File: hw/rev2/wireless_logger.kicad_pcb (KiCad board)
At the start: 4 copper layers, 98 parts, among them J1 FCI 10118194, J3 SSD1306_SER, J4 SWD_10PIN, Q1 2N7002P, Q2 2N7002P, U1 MT29FXX01A, U10 CC2541, U11 STM32F40X_BGA176, U2 MAG3110, U3 MMA8452Q, U4 LPS331AP, U5 L3GD20, U6 MCP111T-315, U7 BQ24095, U8 TPS62698, U9 CC1101, X1 FA-128 26.0000MF10Z-W3, X2 9HT10-32.768KBZF-T, X3 FA-128 32.0000MF20X-K3, X4 XRCGB25M000F0L00R0, X5 9HT10-32.768KBZF-T

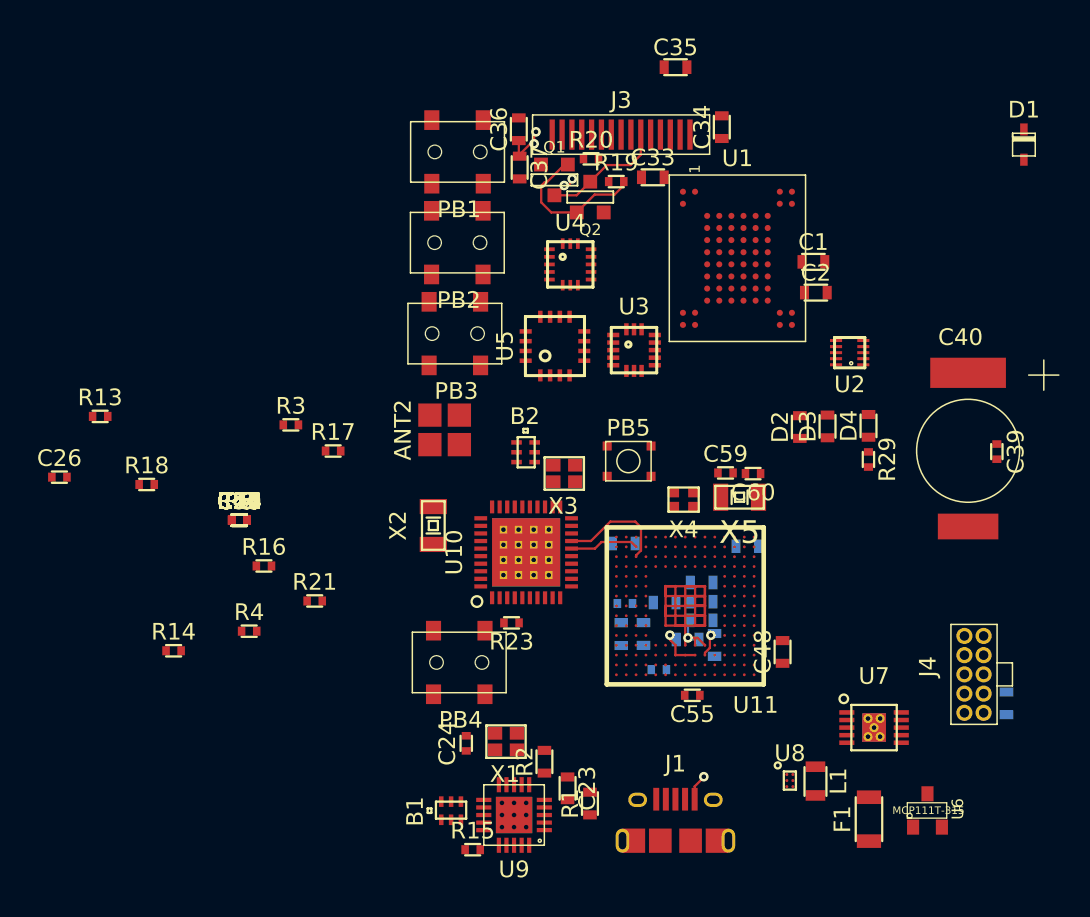
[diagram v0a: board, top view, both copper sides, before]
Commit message: Uhhhh, secondary interconnect assignment and a LOT of routing
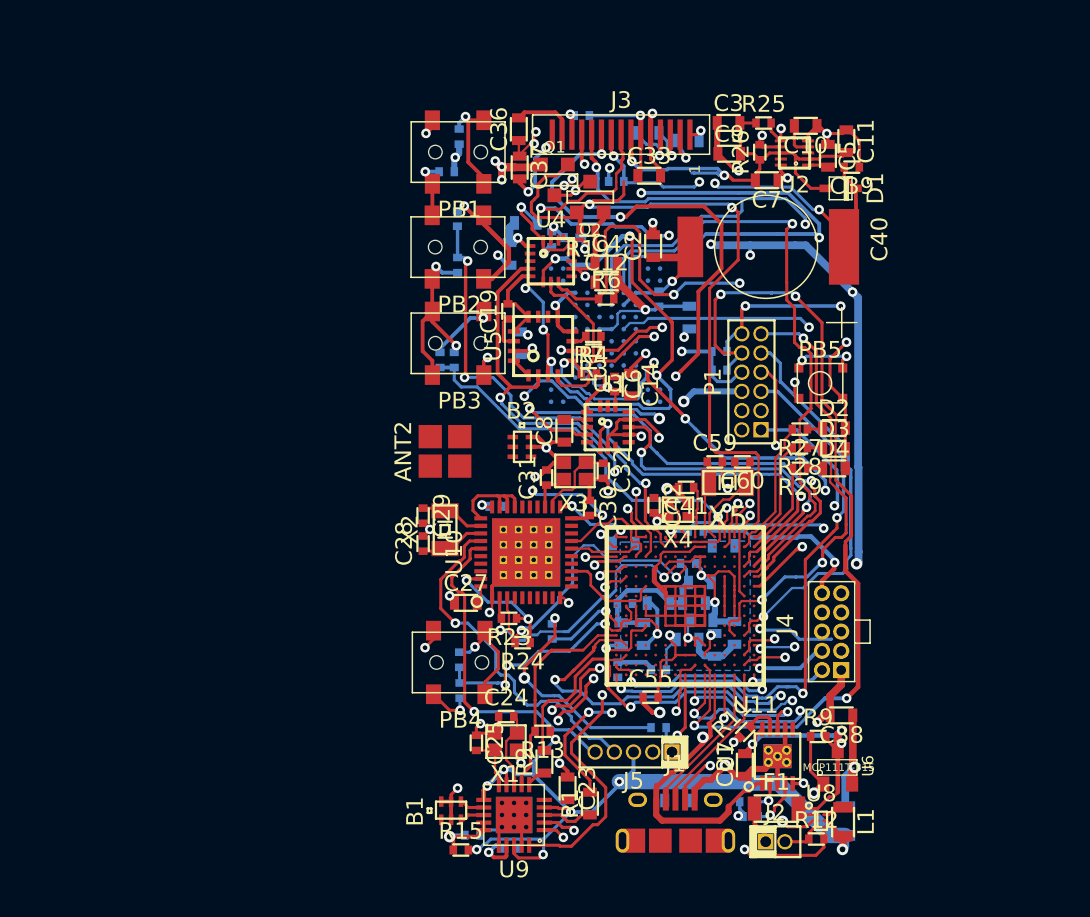
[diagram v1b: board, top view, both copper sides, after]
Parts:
- added C10: 100n, SMD0603, F.Cu at (195.9, 111.4)
- added C11: 100n, SMD0603, F.Cu at (198.6, 112.4)
- added C12: 100n, SMD0603, F.Cu at (182.8, 121.7)
- added C13: 10n, SMD0402, B.Cu at (179.1, 118.9)
- added C14: 2.2u, SMD0603, F.Cu at (184.4, 128.5)
- added C15: 100n, SMD0603, B.Cu at (177.0, 125.7)
- added C16: 100p, SMD0402, B.Cu at (186.2, 122.8)
- added C17: 100n, SMD0603, B.Cu at (177.4, 117.8)
- added C18: 1u, SMD0603, B.Cu at (176.4, 119.8)
- added C19: 10n, SMD0402, F.Cu at (176.2, 123.6)
- added C20: 2.2u, SMD0603, B.Cu at (187.4, 155.9)
- added C21: 2.2u, SMD0603, F.Cu at (191.9, 153.6)
- added C22: 10u, SMD0805, B.Cu at (198.5, 157.3)
- added C27: 1u, SMD0603, F.Cu at (173.5, 142.9)
- added C28: 15p, SMD0402, F.Cu at (170.6, 139.0)
- added C29: 15p, SMD0402, F.Cu at (170.6, 137.1)
- added C3: 2.2u, SMD0603, F.Cu at (190.8, 111.2)
- added C30: 1n, SMD0402, F.Cu at (181.6, 136.6)
- added C31: 12p, SMD0402, F.Cu at (178.8, 134.6)
- added C32: 12p, SMD0402, F.Cu at (182.5, 134.1)
- added C4: 100n, SMD0603, F.Cu at (182.7, 120.5)
- added C5: 100n, SMD0603, F.Cu at (197.4, 113.3)
- added C6: 100p, SMD0402, F.Cu at (183.3, 128.4)
- added C61: 10n, SMD0402, B.Cu at (172.2, 114.4)
- added C62: 10n, SMD0402, B.Cu at (172.9, 120.6)
- added C63: 10n, SMD0402, B.Cu at (172.7, 126.8)
- added C64: 10n, SMD0402, B.Cu at (173.1, 148.7)
- added C7: 1u, SMD0603, F.Cu at (193.3, 115.0)
- added C8: 100n, SMD0603, F.Cu at (180.0, 131.5)
- added C9: 100n, SMD0603, F.Cu at (190.9, 113.2)
- added J2: CONN_2, HDR_2X1_50MIL, F.Cu at (193.9, 158.7)
- added J5: CONN_5, HDR_5X1_50MIL, F.Cu at (184.5, 152.7)
- added P1: CONN_6X2, HDR_6X2_50MIL, F.Cu at (192.3, 128.3)
- added R30: 470k, SMD0402, B.Cu at (173.0, 112.1)
- added R31: 470k, SMD0402, B.Cu at (172.9, 117.5)
- added R32: 470k, SMD0402, B.Cu at (171.8, 126.8)
- added R33: 470k, SMD0402, B.Cu at (173.0, 146.6)
- added R34: 10k, SMD0402, B.Cu at (190.2, 126.3)
- added R35: 10k, SMD0402, B.Cu at (190.2, 127.5)
- C1, C26, C34, C35, C48, C54, C58, R10, R14, R16, R17, R18, R20, R21, R22, R5, R8, U1: moved to B.Cu
- C38: moved to F.Cu
- moved R12 43.6 mm to (196.6, 158.5)
- moved R25 43.5 mm to (193.1, 111.2)
- moved R26 42.1 mm to (192.9, 113.1), turned to 90 degrees
- moved R9 40.8 mm to (196.7, 151.7)
- moved R10 39.0 mm to (192.3, 157.0)
- moved R8 38.4 mm to (192.1, 156.0)
- moved R27 37.5 mm to (195.5, 131.4), turned to 180 degrees
- moved R28 37.3 mm to (195.5, 132.6), turned to 180 degrees
- moved R21 36.6 mm to (181.1, 110.7), turned to 180 degrees
- moved R11 36.2 mm to (191.9, 151.4), turned to 45 degrees
- moved C26 36.1 mm to (173.9, 158.2), turned to 180 degrees
- moved R13 35.9 mm to (178.5, 151.4), turned to 180 degrees
- moved R22 30.2 mm to (188.7, 138.1)
- moved R4 29.9 mm to (181.9, 125.3), turned to 180 degrees
- moved C54 29.8 mm to (188.1, 140.3)
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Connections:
- net N-00000242 renamed /Bluetooth/BT_ANT_DN
- net N-00000243 renamed /Bluetooth/BT_ANT_DP
- net N-00000244 renamed /Bluetooth/BT_ANT_SE
- C1 pad 2: VDD -> V3
- C2 pad 2: VDD -> V3
- C38 pad 2: N-0000078 -> V3
- C45 pad 2: VDD -> V3
- C46 pad 2: VDD -> V3
- C47 pad 2: VDD -> V3
- C48 pad 2: VDD -> V3
- C49 pad 2: VDD -> V3
- C50 pad 2: VDD -> V3
- C51 pad 2: VDD -> V3
- C52 pad 2: VDD -> V3
- C53 pad 2: VDD -> V3
- C54 pad 2: VDD -> V3
- C55 pad 2: VDD -> V3
- C56 pad 2: VDD -> V3
- C57 pad 2: VDD -> V3
- C58 pad 2: VDD -> V3
- D1 pad 1: VDD -> V3
- J3 pad 10: (no net) -> /STM32F4/OLED_nD/C
- J3 pad 7: VDD -> V3
- J3 pad 8: (no net) -> /STM32F4/OLED_nCS
- J4 pad 1: N-0000078 -> V3
- PB1 pad 1: /STM32F4/EXTI5 -> N-0000047
- PB2 pad 1: /STM32F4/EXTI6 -> N-0000046
- PB3 pad 1: /STM32F4/EXTI7 -> N-0000045
- PB4 pad 1: /STM32F4/EXTI8 -> N-0000044
- R13 pad 1: VDD -> V3
- R15 pad 2: VDD -> V3
- R16 pad 1: /STM32F4/BT_NRESET -> /Bluetooth/RF_RESET_N_LOCAL
- R17 pad 1: /STM32F4/BT_NRESET -> /Bluetooth/RF_RESET_N_LOCAL
- R20 pad 1: GND -> /OLED/OLED_GND
- R23 pad 1: VDD -> V3
- R24 pad 1: VDD -> V3
- R25 pad 1: VDD -> V3
- R26 pad 1: VDD -> V3
- R27 pad 2: (no net) -> /STM32F4/LED1
- R28 pad 2: (no net) -> /STM32F4/LED2
- R29 pad 2: (no net) -> /STM32F4/LED3
- R5 pad 1: VDD -> V3
- R6 pad 2: VDD -> V3
- R7 pad 2: VDD -> V3
- U1 pad D3: VDD -> V3
- U1 pad G5: VDD -> V3
- U1 pad G6: VDD -> V3
- U1 pad J8: VDD -> V3
- U1 pad K7: (no net) -> /STM32F4/FLASH_nCS
- U10 pad 10: VDD -> V3
- U10 pad 13: (no net) -> /STM32F4/EXTI2
- U10 pad 20: /STM32F4/BT_NRESET -> /Bluetooth/RF_RESET_N_LOCAL
- U10 pad 21: VDD -> V3
- U10 pad 24: VDD -> V3
- U10 pad 27: VDD -> V3
- U10 pad 28: VDD -> V3
- U10 pad 29: VDD -> V3
- U10 pad 31: VDD -> V3
- U10 pad 39: VDD -> V3
- U10 pad GND: (no net) -> GND
- U11 pad A1: (no net) -> /STM32F4/LED2
- U11 pad A2: (no net) -> /STM32F4/LED3
- U11 pad A4: (no net) -> /Sensors/ACC_INT1
- U11 pad A6: (no net) -> /STM32F4/GYRO_nCS
- U11 pad B1: (no net) -> /OLED/EN
- U11 pad B11: (no net) -> /STM32F4/UART2_RX
- U11 pad B2: (no net) -> /STM32F4/LED1
- U11 pad B5: (no net) -> /STM32F4/FLASH_nCS
- U11 pad B7: (no net) -> /Sensors/PRS_SPI_nCS
- U11 pad C11: (no net) -> /STM32F4/UART2_TX
- U11 pad C5: VDD -> V3
- U11 pad C6: VDD -> V3
- U11 pad C7: VDD -> V3
- U11 pad C8: VDD -> V3
- U11 pad C9: VDD -> V3
- U11 pad D1: (no net) -> /STM32F4/OLED_nCS
- U11 pad D2: (no net) -> /STM32F4/OLED_nRES
- U11 pad F14: (no net) -> /STM32F4/I2C3_SDA
- U11 pad F15: (no net) -> /STM32F4/I2C3_SCL
- U11 pad F3: VDD -> V3
- U11 pad G13: VDD -> V3
- U11 pad G14: (no net) -> /STM32F4/REG_nUSB_CONN
- U11 pad G15: (no net) -> /STM32F4/REG_nCHG
- U11 pad G3: VDD -> V3
- U11 pad H13: VDD -> V3
- U11 pad H15: (no net) -> /Power/MODE
- U11 pad J12: VDD -> V3
- U11 pad J13: VDD -> V3
- U11 pad K1: (no net) -> /STM32F4/EXTI7
- U11 pad K4: VDD -> V3
- U11 pad M3: (no net) -> /STM32F4/EXTI1
- U11 pad M6: (no net) -> /STM32F4/EXTI2
- U11 pad N10: VDD -> V3
- U11 pad N8: VDD -> V3
- U11 pad N9: VDD -> V3
- U11 pad P1: VDD -> V3
- U11 pad P12: (no net) -> /STM32F4/SPI2_NSS
- U11 pad R1: VDD -> V3
- U11 pad R10: (no net) -> /STM32F4/BT_NRESET
- U11 pad R11: (no net) -> /STM32F4/CC1101_nCS
- U11 pad R15: (no net) -> /STM32F4/SPI2_MOSI
- U11 pad R2: (no net) -> /STM32F4/OLED_nD/C
- U11 pad R8: /STM32F4/EXTI7 -> (no net)
- U2 pad 2: VDD -> V3
- U2 pad 8: VDD -> V3
- U3 pad 1: VDD -> V3
- U3 pad 11: (no net) -> /Sensors/ACC_INT1
- U3 pad 14: VDD -> V3
- U4 pad 1: VDD -> V3
- U4 pad 14: VDD -> V3
- U5 pad 1: VDD -> V3
- U5 pad 15: VDD -> V3
- U5 pad 16: VDD -> V3
- U7 pad 5: (no net) -> /STM32F4/REG_nUSB_CONN
- U7 pad 8: (no net) -> /STM32F4/REG_nCHG
- U7 pad GND: (no net) -> GND
- U8 pad 3: (no net) -> GND
- U9 pad 11: VDD -> V3
- U9 pad 18: VDD -> V3
- U9 pad 4: VDD -> V3
- U9 pad 9: VDD -> V3
- X1 pad GND: (no net) -> GND
- X3 pad GND: (no net) -> GND
- X4 pad GND: (no net) -> GND
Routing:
- net V3: track 0.00 -> 273.7 mm, vias 0 -> 27
- net GND: track 46.1 -> 245.8 mm, vias 2 -> 45
- net Vbat: track 0.00 -> 92.0 mm, vias 0 -> 8
- net /Sensors/GYR_SPI_MOSI: track 0.00 -> 82.8 mm, vias 0 -> 8
- net /OLED/SDIN: track 0.00 -> 68.9 mm, vias 0 -> 5
- net /Sensors/ACC_I2C_SCL: track 0.00 -> 66.0 mm, vias 0 -> 3
- net /OLED/SCLK: track 0.00 -> 64.7 mm, vias 0 -> 3
- net /Sensors/GYR_SPI_MISO: track 0.00 -> 59.5 mm, vias 0 -> 5
- net /STM32F4/I2C3_SDA: track 0.00 -> 56.6 mm, vias 0 -> 4
- net /Sensors/GYR_SPI_CLK: track 0.00 -> 56.4 mm, vias 0 -> 6
- net /STM32F4/I2C3_SCL: track 0.00 -> 55.9 mm, vias 0 -> 4
- net /Sensors/ACC_I2C_SDA: track 0.00 -> 53.2 mm, vias 0 -> 3
- net Vbus: track 0.00 -> 50.8 mm, vias 0 -> 2
- net /STM32F4/SPI2_CLK: track 0.00 -> 49.3 mm, vias 0 -> 3
- net /STM32F4/SPI2_NSS: track 0.00 -> 48.6 mm, vias 0 -> 3
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- added copper zone on GND_PLANE, net /OLED/OLED_GND
- added copper zone on B.Cu, net GND
- added copper zone on GND_PLANE, net GND
- added copper zone on Inner2.Cu, net V3
- removed copper zone on GND, net /OLED/OLED_GND
- removed copper zone on GND, net GND
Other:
- net class 50OHM added: clearance 0.1524, trace_width 0.2032, via_dia 0.635, via_drill 0.3048
- net class Default: trace_width 0.2032 -> 0.1524
